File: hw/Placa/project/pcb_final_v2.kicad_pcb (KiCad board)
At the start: 2 copper layers, 50.7 x 80 mm, 21 parts, among them J1 pin_socket-bluepill, J10 tcrt5000_conector_2, J11 tcrt5000_conector_3, J12 tcrt5000_conector_1, J2 pin_socket-bluepill, J9 tof-connector_3, SW2 key, U2 Receptor IR, U4 AMS1117-3.3

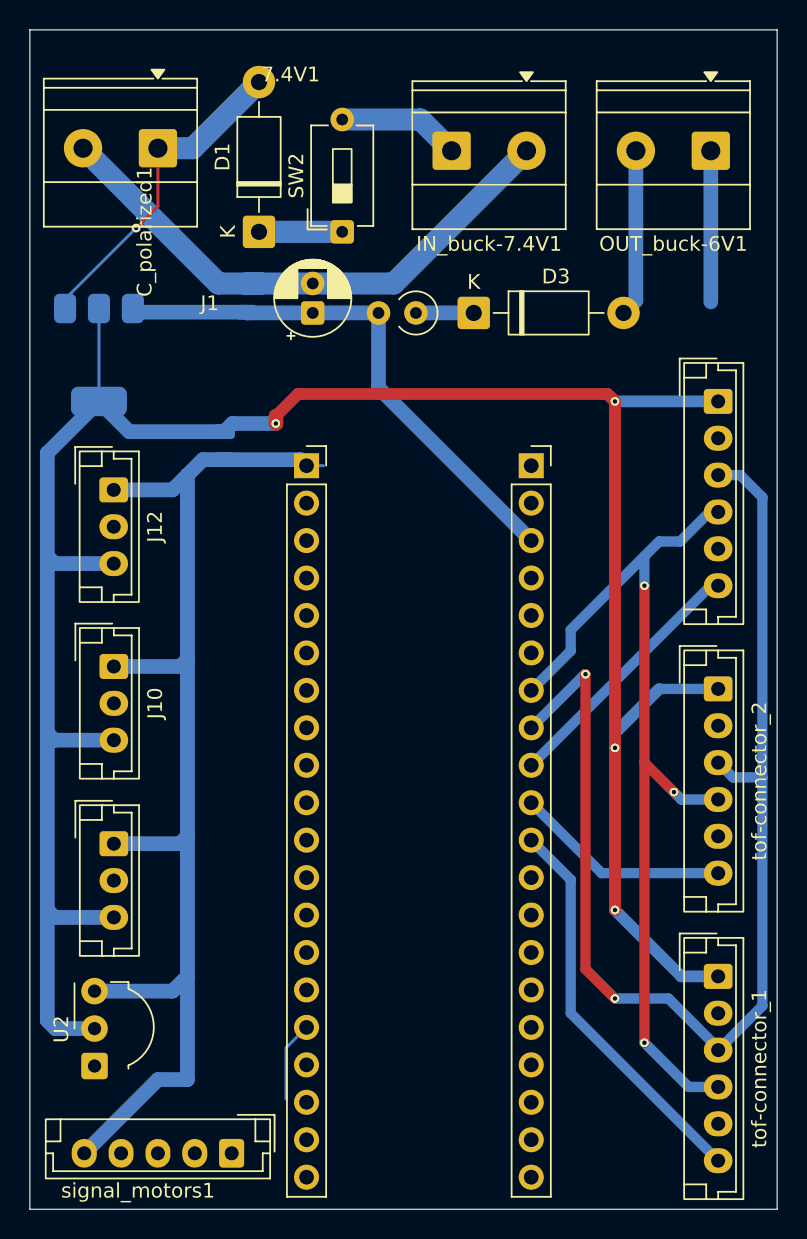
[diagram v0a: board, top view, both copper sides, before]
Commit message: pcb finalizada
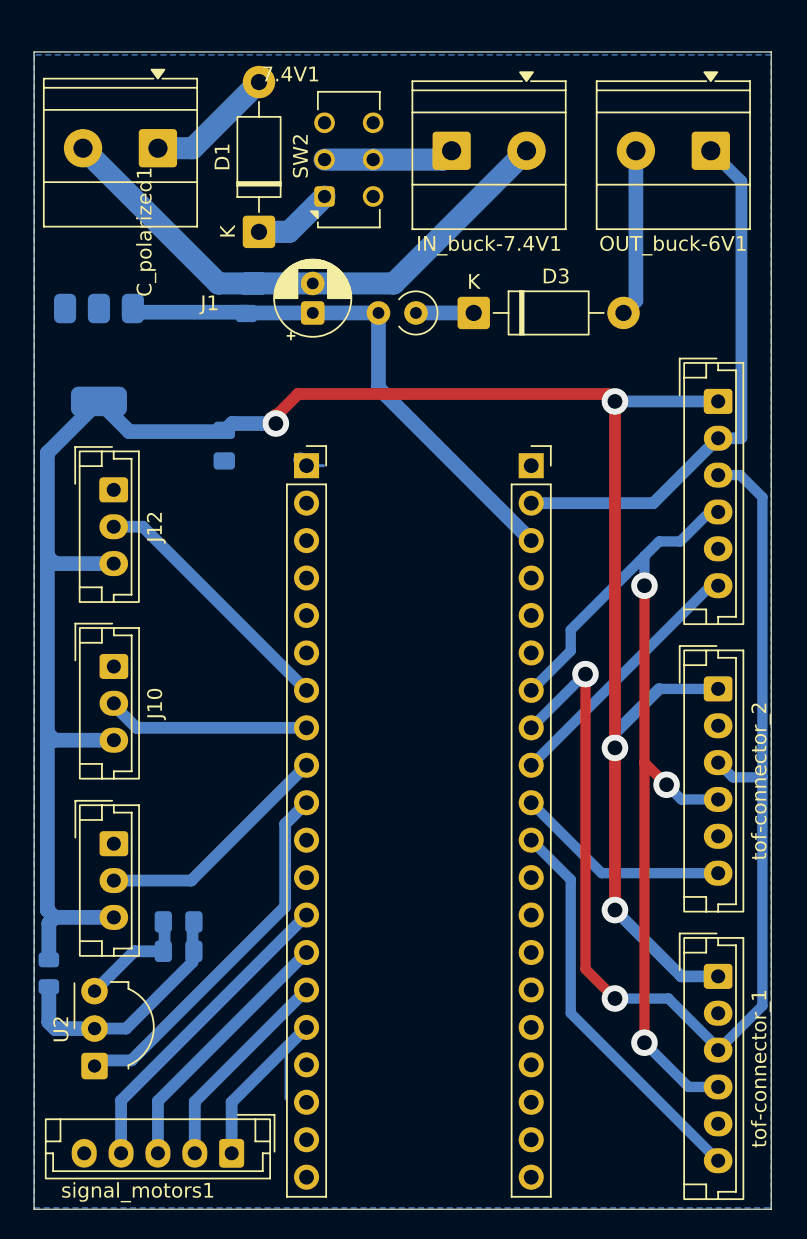
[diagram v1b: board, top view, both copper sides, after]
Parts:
- added C1: 4,7uF, Capacitor_SMD:C_0805_2012Metric_Pad1.18x1.45mm_HandSolder, B.Cu at (123.4, 112.8)
- added C4: 100nF, Capacitor_SMD:C_0805_2012Metric_Pad1.18x1.45mm_HandSolder, B.Cu at (123.4, 110.8)
- added R1: 100, Resistor_SMD:R_0805_2012Metric, B.Cu at (114.6, 114.3)
- C2, C3: footprint Capacitor_SMD:C_0805_2012Metric -> Capacitor_SMD:C_0805_2012Metric_Pad1.18x1.45mm_HandSolder
- SW2: footprint Button_Switch_THT:SW_DIP_SPSTx01_Slide_6.7x4.1mm_W7.62mm_P2.54mm_LowProfile -> Button_Switch_THT:SW_CK_JS202011CQN_DPDT_Straight
- moved SW2 2.68 mm to (133.3, 61.6)
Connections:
- 7.4V1 pad 1: +7.4V -> Net-(7.4V1-Pin_1)
- C2 pad 1: GNDPWR -> +5V
- C2 pad 2: +5V -> GNDPWR
- D1 pad 2: +7.4V -> Net-(7.4V1-Pin_1)
- IN_buck-7.4V1 pad 2: IN-BUCK -> +7.4V
- SW2 pad 2: IN-BUCK -> +7.4V
- U4 pad 1: +7.4V -> (no net)
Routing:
- net GNDS: track 92.7 -> 46.0 mm
- net D4: track 0.00 -> 25.1 mm
- net MB-: track 0.00 -> 21.4 mm
- net MB+: track 0.00 -> 17.8 mm
- net D1: track 0.00 -> 17.7 mm
- net D3: track 0.00 -> 16.3 mm
- net MA-: track 0.00 -> 14.2 mm
- net D2: track 0.72 -> 14.5 mm
- net +7.4V: track 22.2 -> 8.87 mm, vias 1 -> 0
- net MA+: track 5.43 -> 16.1 mm
- net Net-(7.4V1-Pin_1): track 0.00 -> 8.71 mm
- net IN-BUCK: track 8.30 -> 0.00 mm
- net +3V3: track 164.7 -> 167.4 mm
- added copper zone on B.Cu, net GNDS
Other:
- board size 50.7 x 80 mm -> 50 x 78.5 mm
